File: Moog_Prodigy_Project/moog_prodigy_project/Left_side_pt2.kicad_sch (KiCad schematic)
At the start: 64 parts, among them J7 Conn_01x02_Socket, Q4 BC107, Q7 BC549, SW3 Switch_4x4, SW4 SW_Slide_DPDT_3x3, SW5 Switch_4x4, U2B2 OPA134, U4B1 OPA134, U6 NE5532, U7 NE5532, U8 LT1011CN8

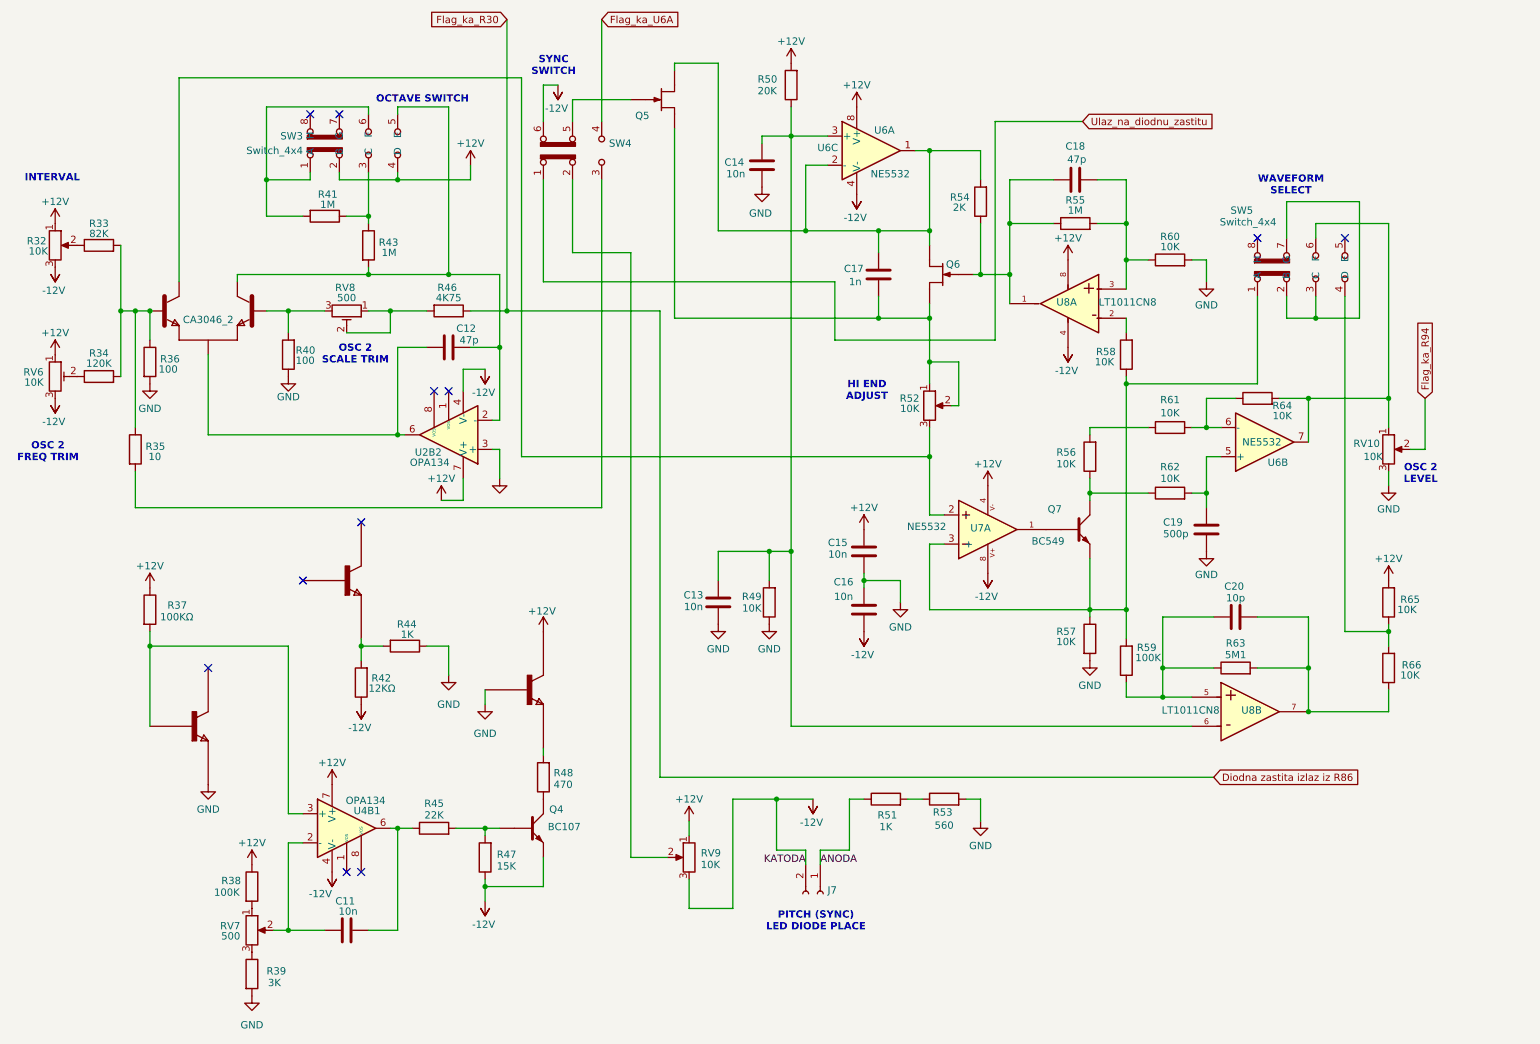
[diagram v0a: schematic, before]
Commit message: Latest checkpoints update 05.06.2026
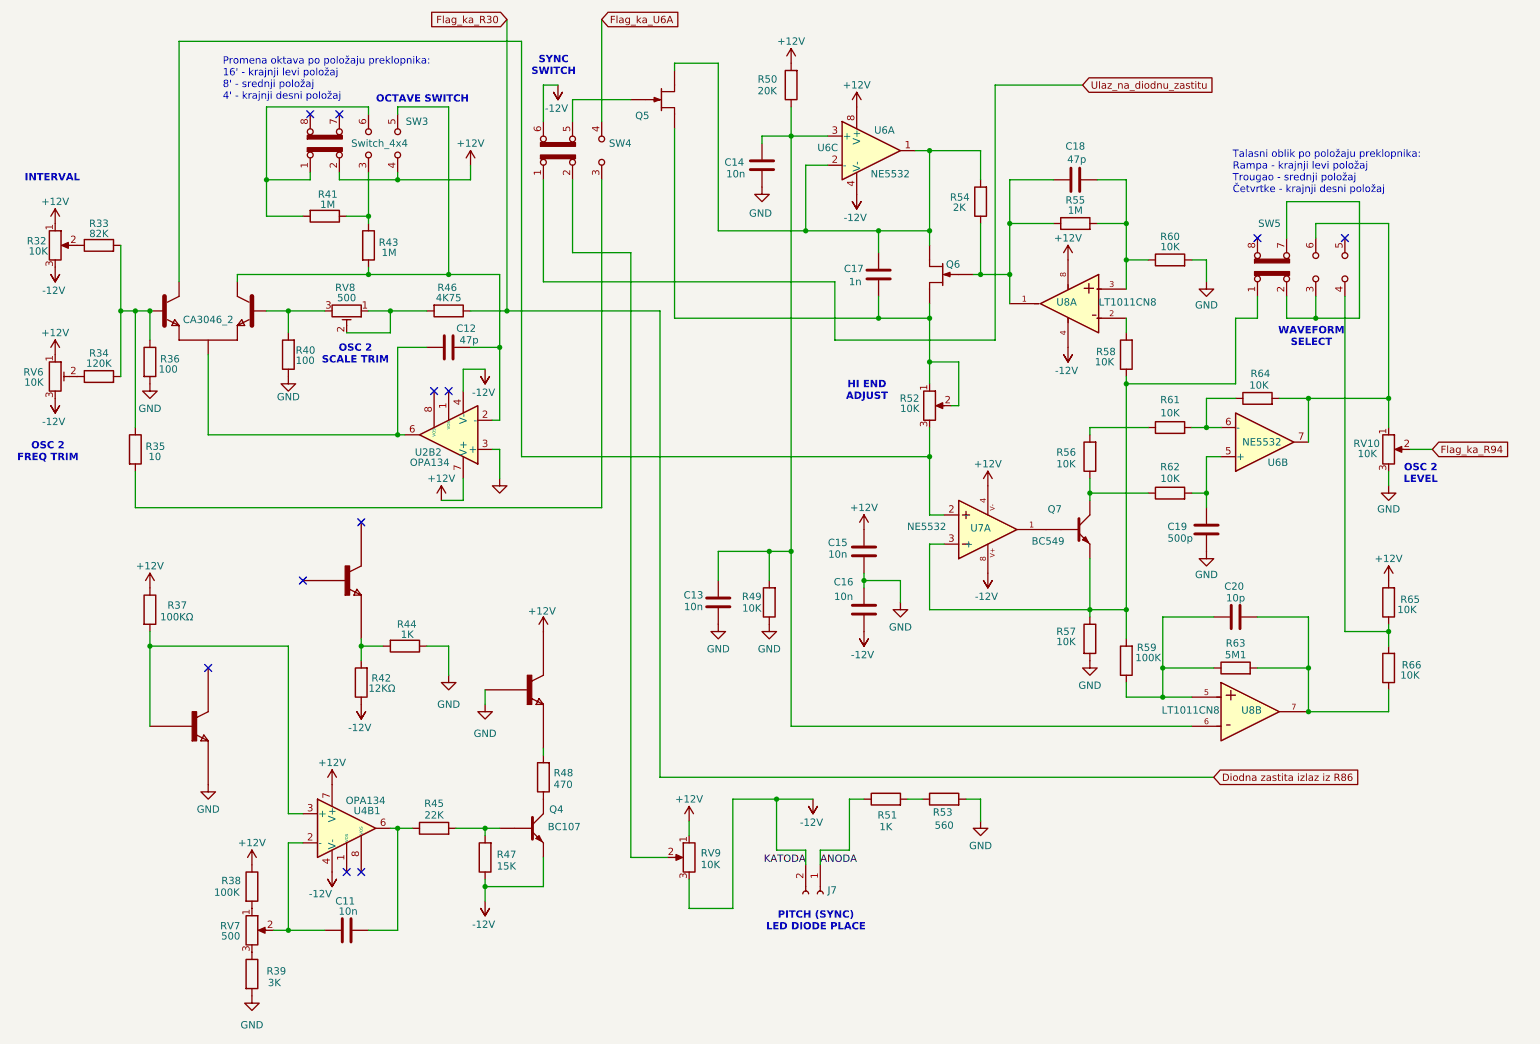
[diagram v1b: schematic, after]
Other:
- note added: "Promena oktava po položaju preklopnika: 16' - krajnji levi položaj 8' - srednji položaj 4' - krajnji desni položaj"
- note added: "Talasni oblik po položaju preklopnika: Rampa - krajnji levi položaj Trougao - srednji položaj Četvrtke - krajnji desni položaj"
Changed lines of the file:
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@@
 	(text "WAVEFORM\nSELECT"
 		(exclude_from_sim no)
-		(at 242.062 45.466 0)
+		(at 245.618 71.882 0)
 		(effects
 			(font
@@
 		)
 	)
+	(text "Talasni oblik po položaju preklopnika:\nRampa - krajnji levi položaj\nTrougao - srednji položaj\nČetvrtke - krajnji desni položaj\n"
+		(exclude_from_sim no)
+		(at 231.902 43.18 0)
+		(effects
+			(font
+				(size 1.27 1.27)
+			)
+			(justify left)
+		)
+	)
 	(text "INTERVAL"
 		(exclude_from_sim no)
@@
 		)
 	)
+	(text "Promena oktava po položaju preklopnika:\n16' - krajnji levi položaj \n8' - srednji položaj \n4' - krajnji desni položaj \n"
+		(exclude_from_sim no)
+		(at 55.88 26.924 0)
+		(effects
+			(font
+				(size 1.27 1.27)
+			)
+			(justify left)
+		)
+	)
 	(text "HI END \nADJUST"
 		(exclude_from_sim no)
@@
 	(wire
 		(pts
-			(xy 190.5 72.39) (xy 190.5 34.29)
+			(xy 190.5 72.39) (xy 190.5 27.94)
 		)
 		(stroke
@@
 	(wire
 		(pts
-			(xy 265.43 91.44) (xy 265.43 82.55)
-		)
-		(stroke
-			(width 0)
-			(type default)
-		)
-	)
-	(wire
-		(pts
-			(xy 48.26 62.23) (xy 48.26 26.67)
+			(xy 48.26 62.23) (xy 48.26 20.32)
 		)
 		(stroke
@@
 	(wire
 		(pts
-			(xy 48.26 26.67) (xy 107.95 26.67)
+			(xy 48.26 20.32) (xy 107.95 20.32)
 		)
 		(stroke
@@
 	(wire
 		(pts
-			(xy 236.22 64.77) (xy 236.22 80.01)
+			(xy 232.41 68.58) (xy 232.41 80.01)
 		)
 		(stroke
@@
 	(wire
 		(pts
-			(xy 262.89 91.44) (xy 265.43 91.44)
+			(xy 262.89 91.44) (xy 266.7 91.44)
 		)
 		(stroke
@@
 	(wire
 		(pts
-			(xy 190.5 34.29) (xy 205.74 34.29)
+			(xy 190.5 27.94) (xy 205.74 27.94)
 		)
 		(stroke
@@
 	(wire
 		(pts
-			(xy 107.95 26.67) (xy 107.95 92.71)
+			(xy 107.95 20.32) (xy 107.95 92.71)
 		)
 		(stroke
@@
 	(wire
 		(pts
+			(xy 232.41 68.58) (xy 236.22 68.58)
+		)
+		(stroke
+			(width 0)
+			(type default)
+		)
+	)
+	(wire
+		(pts
 			(xy 208.28 52.07) (xy 213.36 52.07)
 		)
@@
 	(wire
 		(pts
+			(xy 236.22 68.58) (xy 236.22 64.77)
+		)
+		(stroke
+			(width 0)
+			(type default)
+		)
+	)
+	(wire
+		(pts
 			(xy 158.75 152.4) (xy 152.4 152.4)
 		)
@@
 	(wire
 		(pts
-			(xy 213.36 80.01) (xy 236.22 80.01)
+			(xy 213.36 80.01) (xy 232.41 80.01)
 		)
 		(stroke
@@
 	(global_label "Ulaz_na_diodnu_zastitu"
 		(shape input)
-		(at 205.74 34.29 0)
+		(at 205.74 27.94 0)
 		(fields_autoplaced yes)
 		(effects
@@
 		)
 		(property "Intersheetrefs" "${INTERSHEET_REFS}"
-			(at 230.859 34.29 0)
+			(at 230.859 27.94 0)
 			(effects
 				(font
@@
 	(global_label "Flag_ka_R94"
 		(shape input)
-		(at 265.43 82.55 90)
+		(at 266.7 91.44 0)
 		(fields_autoplaced yes)
 		(effects
@@
 		)
 		(property "Intersheetrefs" "${INTERSHEET_REFS}"
-			(at 265.43 67.7117 90)
+			(at 281.5383 91.44 0)
 			(effects
 				(font
@@
 		)
 		(property "Value" "10K"
-			(at 258.064 92.71 0)
+			(at 257.048 92.202 0)
 			(effects
 				(font
@@
 		(dnp no)
 		(property "Reference" "R64"
-			(at 240.538 83.82 90)
+			(at 236.728 78.232 90)
 			(effects
 				(font
@@
 		)
 		(property "Value" "10K"
-			(at 240.538 85.598 90)
+			(at 236.474 80.264 90)
 			(effects
 				(font
@@
 	)
 	(symbol
+		(lib_name "SW_Slide_DPDT_4x4_1")
 		(lib_id "Power_supply:SW_Slide_DPDT_4x4")
 		(at 78.74 36.83 0)
@@
 		(on_board yes)
 		(dnp no)
-		(fields_autoplaced yes)
 		(property "Reference" "SW3"
-			(at 69.85 36.8299 0)
+			(at 91.694 34.29 0)
 			(effects
 				(font
@@
 		)
 		(property "Value" "Switch_4x4"
-			(at 69.85 39.3699 0)
+			(at 88.138 38.1 0)
 			(effects
 				(font
@@
 		(dnp no)
 		(property "Reference" "SW5"
-			(at 235.458 49.784 0)
+			(at 240.284 52.07 0)
 			(effects
 				(font
@@
 		)
 		(property "Value" "Switch_4x4"
-			(at 239.522 51.816 0)
+			(at 252.73 50.292 0)
 			(effects
 				(font
@@
 				)
 				(justify right)
+				(hide yes)
 			)
 		)
@@
 		(dnp no)
 		(property "Reference" "C19"
-			(at 221.488 104.14 0)
+			(at 222.25 104.902 0)
 			(effects
 				(font
@@
 		)
 		(property "Value" "500p"
-			(at 221.996 106.172 0)
+			(at 222.758 106.934 0)
 			(effects
 				(font
